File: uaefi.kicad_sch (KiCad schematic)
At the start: 68 parts, among them J1 Conn_02x02_Odd_Even, J1 USB_B_Mini, J1 USB_C, J10 5569-16A2, J11 Conn_02x02_Odd_Even, J12 Conn_02x02_Odd_Even, J13 Conn_02x02_Odd_Even, J14 Conn_02x02_Odd_Even, J15 Conn_02x02_Odd_Even, J16 Conn_02x02_Odd_Even, J17 Conn_01x06, J17 Conn_02x02_Odd_Even, J18 Conn_02x02_Odd_Even, J19 Conn_02x02_Odd_Even, J2 5569-20A2, J20 Conn_02x02_Odd_Even, J21 Conn_02x02_Odd_Even, J22 Conn_02x02_Odd_Even, J24 Conn_02x02_Odd_Even, J3 5569-06A2, J4 5569-08A2, J5 5569-18A2, J5 Conn_01x05_Male, M1 Module-power_12and5V-0.3, M3 Module-knock-0.2, M3 Module-vr-discrete-0.5, M4 Module-vr-max9924-0.1, M5 Module-wbo-0.5, M6 Module:mega-mcu100/0.3, M7 Module-can-0.1, P1 Pad, P2 Pad, P3 Pad, P4 Pad, P5 Pad, P6 Pad, P7 Pad, P8 Pad, U4 JDY-33

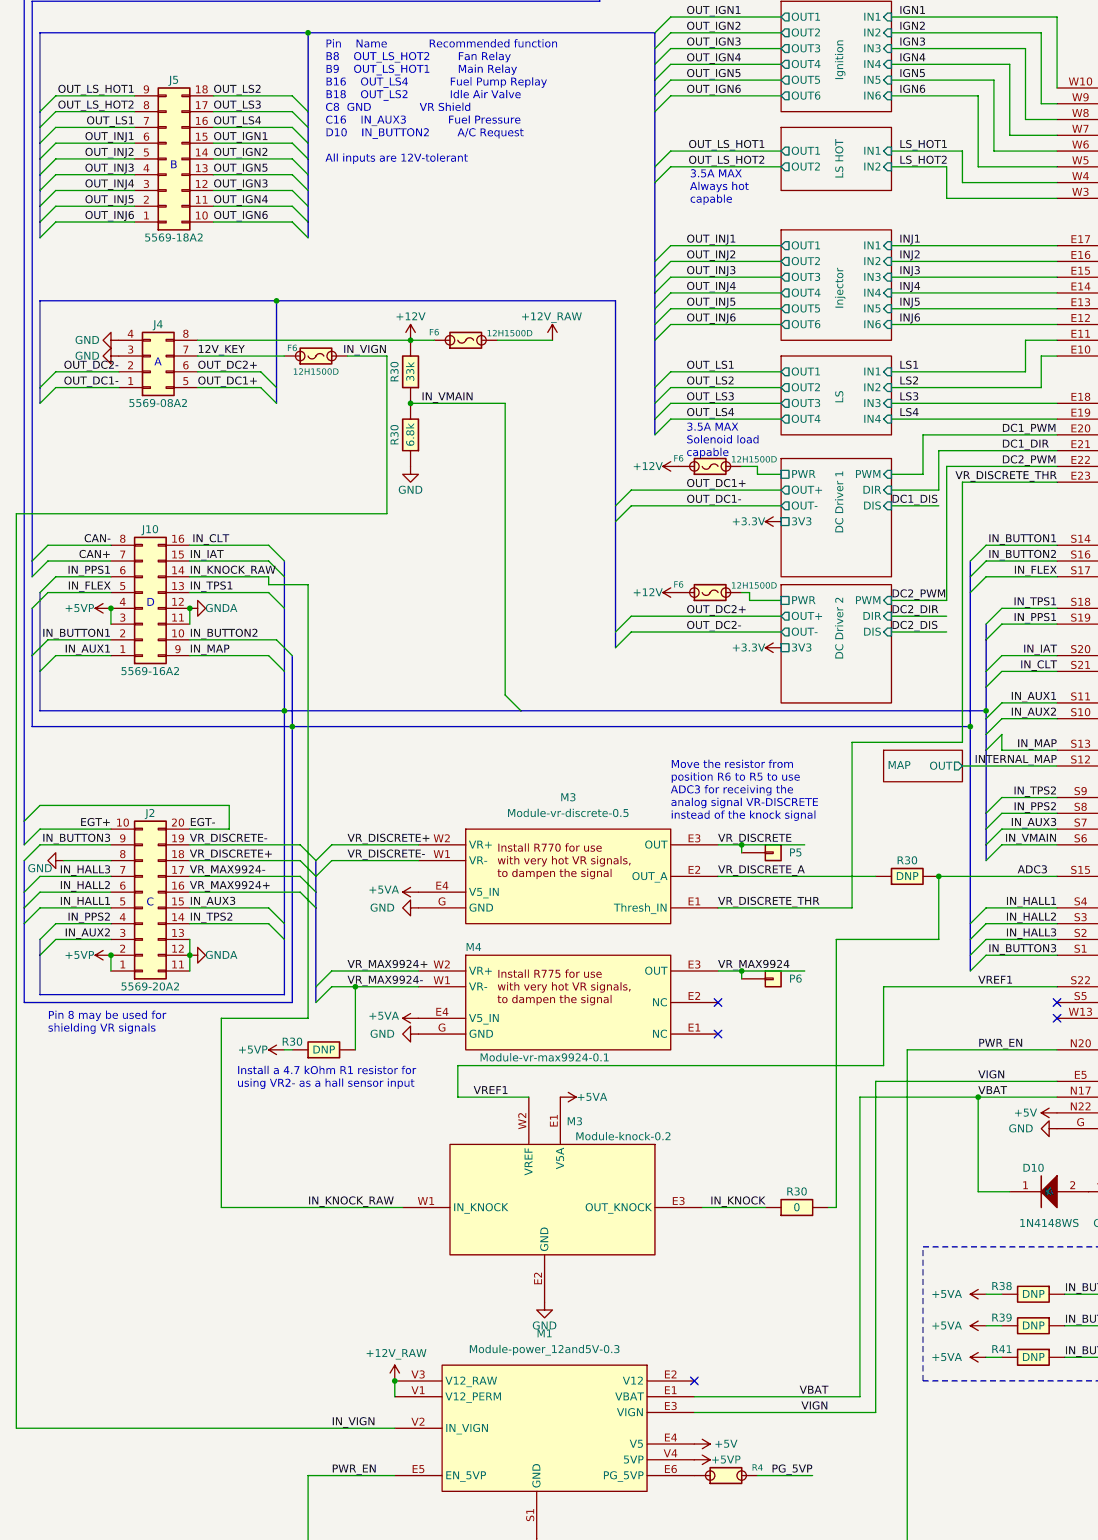
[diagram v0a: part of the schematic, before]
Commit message: #81 #82 #86 #87
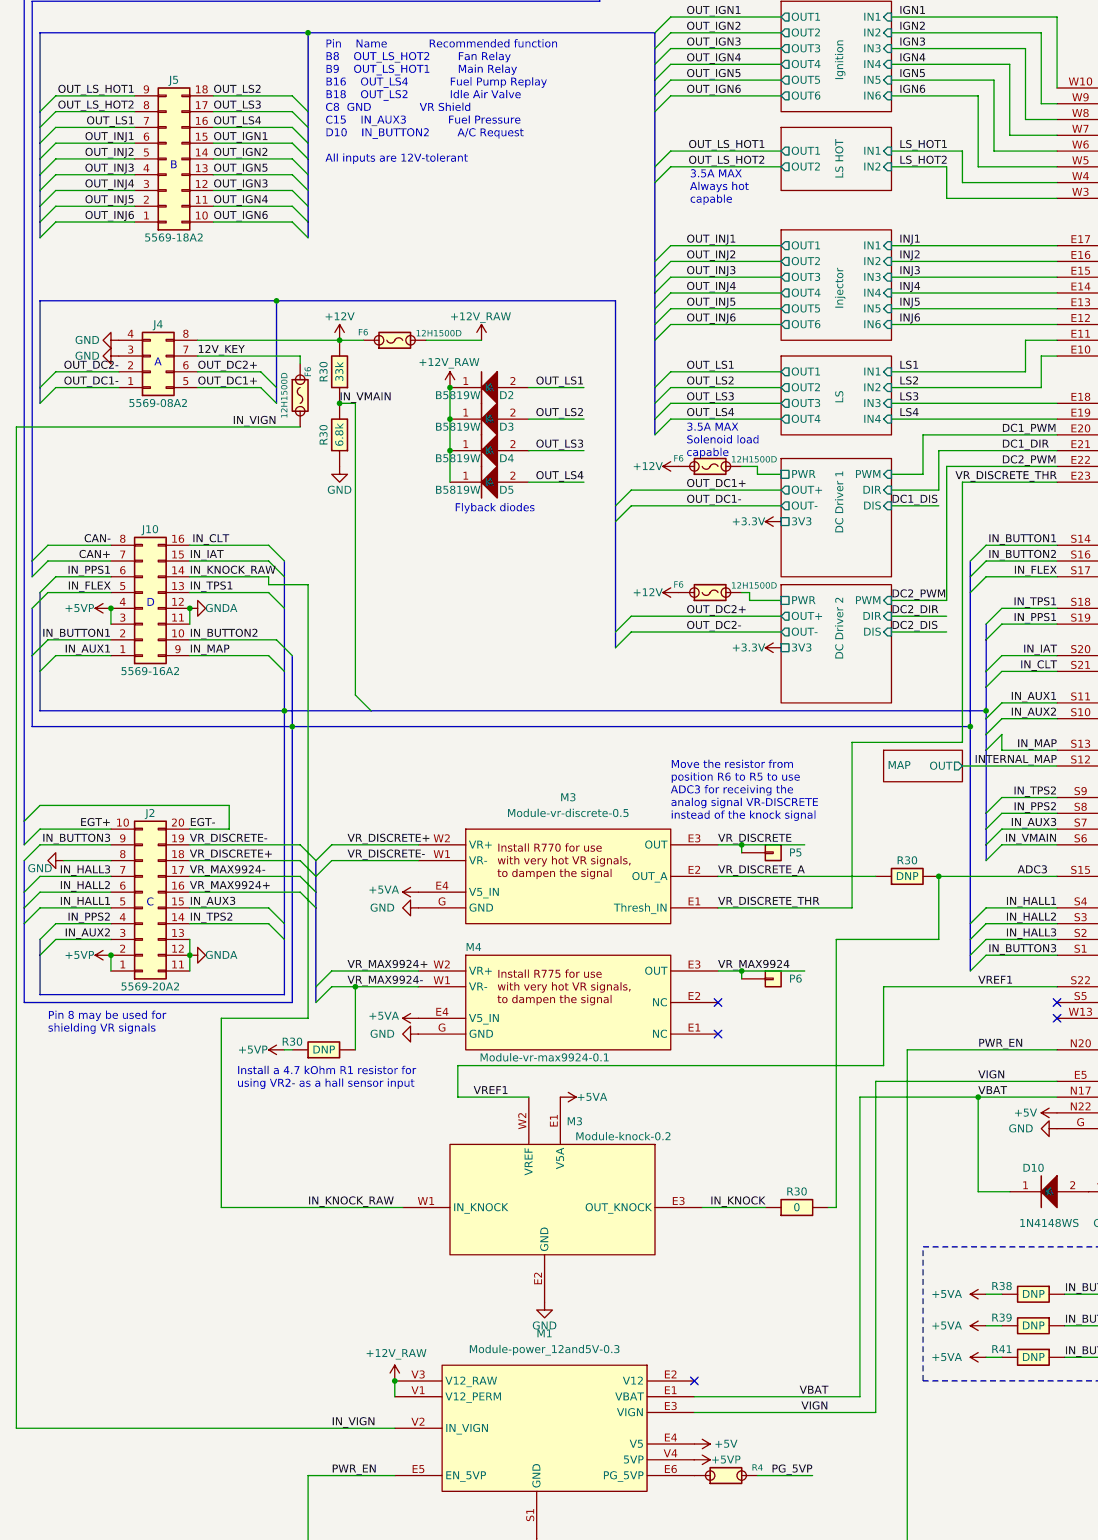
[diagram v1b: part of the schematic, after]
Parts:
- added D2, D3, D4, D5: B5819W, hellen-one-common:SOD-123, symbol hellen-one-common:1N4148WS
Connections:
- net +12V_RAW: now also D2.1 (K), D3.1 (K), D4.1 (K), D5.1 (K)
- net OUT_LS1: now also D2.2 (A)
- net OUT_LS2: now also D3.2 (A)
- net OUT_LS3: now also D4.2 (A)
- net OUT_LS4: now also D5.2 (A)
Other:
- note added: "Flyback diodes"
- note added: "Pin Name Recommended function B8 OUT_LS_HOT2 Fan Relay B9 OUT_LS_HOT1 Main Relay B16 OUT_LS4 Fuel Pump Replay B18 OUT_LS2 Idle Air Valve C8 GND VR Shield C15 IN_AUX3 Fuel Pressure D10 IN_BUTTON2 A/C Request All inputs are 12V-tolerant"
- note removed: "Pin Name Recommended function B8 OUT_LS_HOT2 Fan Relay B9 OUT_LS_HOT1 Main Relay B16 OUT_LS4 Fuel Pump Replay B18 OUT_LS2 Idle Air Valve C8 GND VR Shield C16 IN_AUX3 Fuel Pressure D10 IN_BUTTON2 A/C Request All inputs are 12V-tolerant"
- moved on the sheet: F6, R30
